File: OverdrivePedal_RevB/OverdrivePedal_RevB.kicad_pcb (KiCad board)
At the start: 2 copper layers, 26.7 x 34.9 mm, 25 parts, among them J1 Conn_01x02, J2 Conn_01x02, J3 Conn_01x03, J4 Conn_01x03, J5 Conn_01x03, J6 Conn_01x02, U2 TL071, U3 TPS60400, U4 KIA78L05T, U5 XC6902N501PR-G

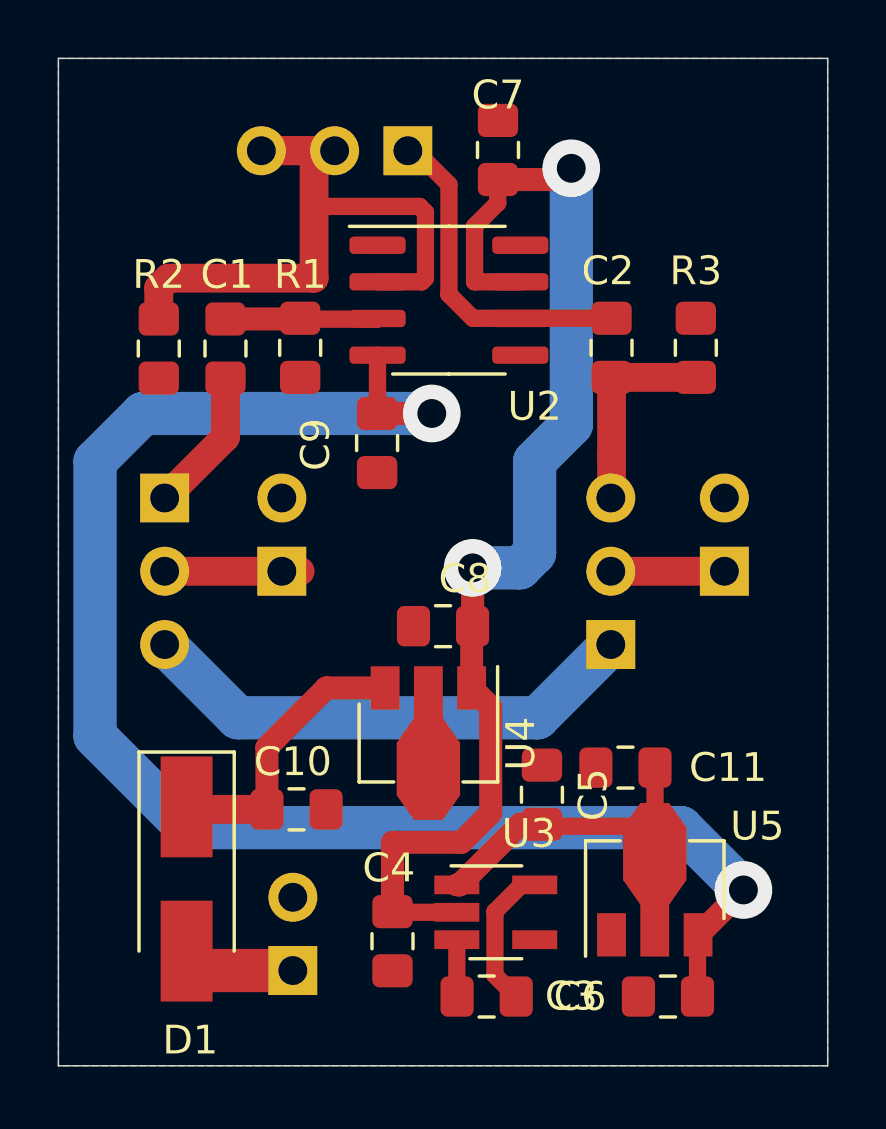
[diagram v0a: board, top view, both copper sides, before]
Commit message: updated revb
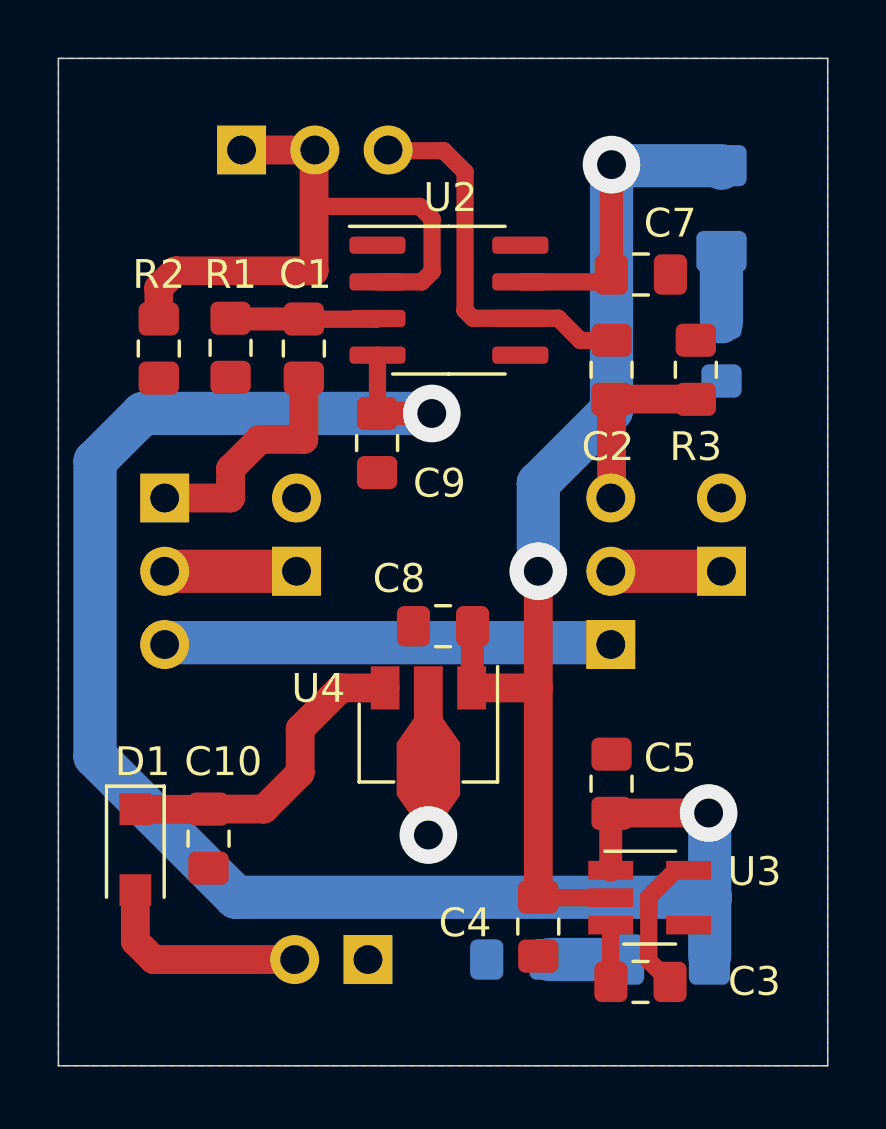
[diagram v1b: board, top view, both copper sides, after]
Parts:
- removed C11, C6: 1uF, Capacitor_SMD:C_0805_2012Metric_Pad1.15x1.40mm_HandSolder
- removed J4: Conn_01x03, Connector_PinHeader_2.54mm:PinHeader_1x03_P2.54mm_Vertical
- removed U5: XC6902N501PR-G, Package_TO_SOT_SMD:SOT-89-3
- added D2: LED, LED_SMD:LED_1206_3216Metric_Pad1.42x1.75mm_HandSolder, B.Cu at (80.1, 198.9)
- added D3: LED, LED_SMD:LED_1206_3216Metric_Pad1.42x1.75mm_HandSolder, B.Cu at (82.0, 172.8)
- added R6: 1K, Resistor_SMD:R_0805_2012Metric_Pad1.15x1.40mm_HandSolder, B.Cu at (74.9, 198.9)
- added R9: 1K, Resistor_SMD:R_0805_2012Metric_Pad1.15x1.40mm_HandSolder, B.Cu at (82.0, 177.8)
- added RV1: B10K, Connector_PinHeader_2.54mm:PinHeader_1x03_P2.54mm_Vertical, B.Cu at (65.4, 170.8)
- D1: value D_Schottky -> BYS12-90; footprint Diode_SMD:D_SMA_Handsoldering -> Diode_SMD:D_SOD-123F
- J1, J6: value Conn_01x02 -> AudioJack2
- J2: value Conn_01x02 -> Barrel_Jack
- moved C7 6.57 mm to (79.2, 175.1), turned to 0 degrees
- moved U3 5.36 mm to (79.6, 196.7)
- moved C3 5.36 mm to (79.2, 199.7)
- moved C4 5.08 mm to (75.7, 197.7)
- moved C10 3.21 mm to (64.3, 194.7), turned to 270 degrees
- moved C1 2.72 mm to (67.6, 177.7)
- moved J2 2.63 mm to (69.8, 198.9), turned to 90 degrees
- moved C5 2.44 mm to (78.2, 192.8)
- moved R1 2.41 mm to (65.0, 177.7)
- moved D1 2.05 mm to (61.7, 195.1)
- moved C2 0.76 mm to (78.2, 178.4)
- moved R3 0.76 mm to (81.2, 178.4)
- moved J1 0.51 mm to (67.3, 185.4)
- moved J6 0.10 mm to (82.0, 185.4)
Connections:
- C5 pad 1: /PosNeg5V_PSU/-5V_POL -> -5V
- J2 pad 1: /PosNeg5V_PSU/+9V_IN -> GNDS
- J2 pad 2: GNDS -> /PosNeg5V_PSU/+9V_IN
- U3 pad 1: /PosNeg5V_PSU/-5V_POL -> -5V
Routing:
- net /PosNeg5V_PSU/-5V_POL: track 13.6 -> 0.00 mm
- net -5V: track 54.9 -> 61.3 mm
- net /PosNeg5V_PSU/+9V_IN: track 3.50 -> 7.56 mm
- net Net-(C1-Pad2): track 5.03 -> 8.39 mm
- net +5V: track 41.6 -> 44.9 mm
- net Net-(D2-Pad2): track 0.00 -> 2.54 mm
- net Net-(D3-Pad1): track 0.00 -> 2.31 mm
- net Net-(J3-Pad3): track 17.6 -> 15.5 mm
- net Net-(R2-Pad1): track 23.3 -> 21.5 mm
- net Net-(C2-Pad2): track 11.7 -> 12.6 mm
- net Net-(C2-Pad1): track 7.00 -> 6.24 mm
- net Net-(J1-Pad1): track 4.06 -> 4.57 mm
- net GNDS: vias 0 -> 1
